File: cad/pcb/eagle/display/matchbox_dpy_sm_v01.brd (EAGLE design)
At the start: 40 x 32 mm, 16 parts, among them J1 DF12-32-DS, J2 DF12-32-DS, SW1 B3U-3100PM-B, U1 LM2750

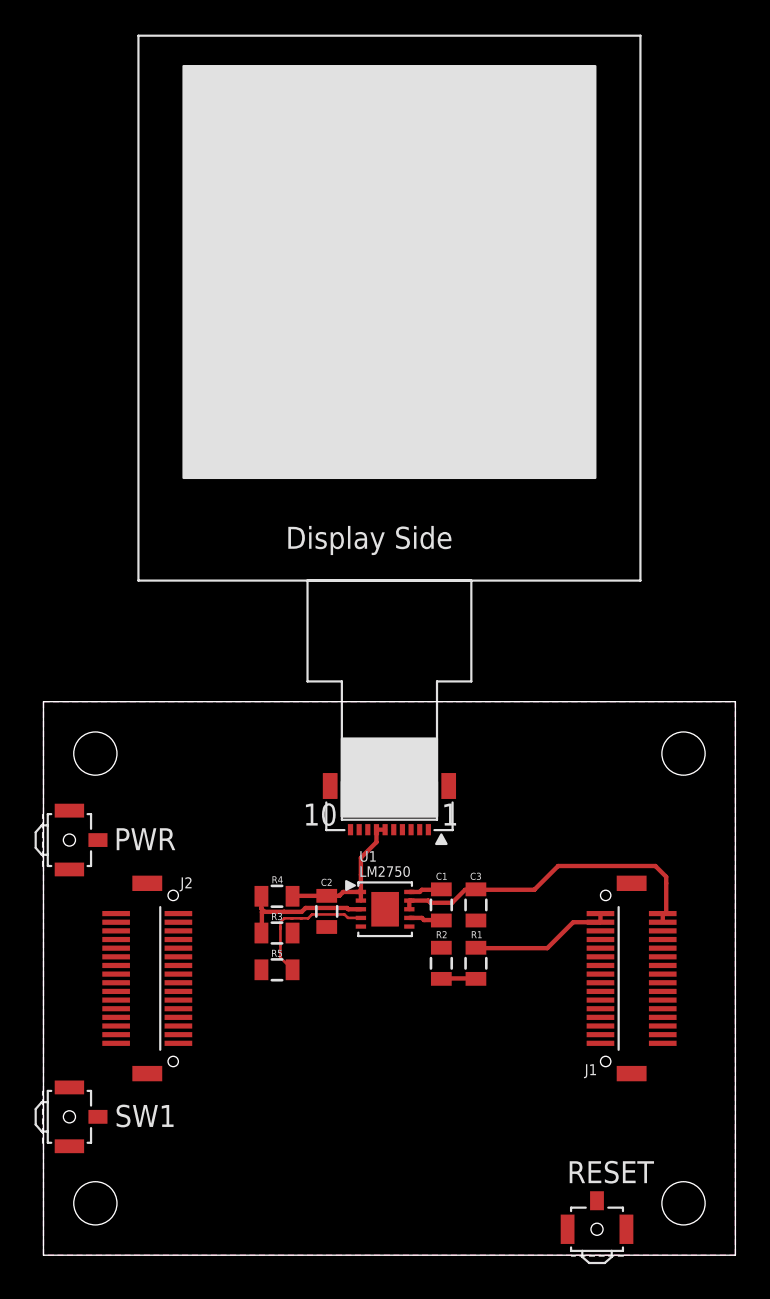
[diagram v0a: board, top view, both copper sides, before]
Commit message: Tweak display board v01
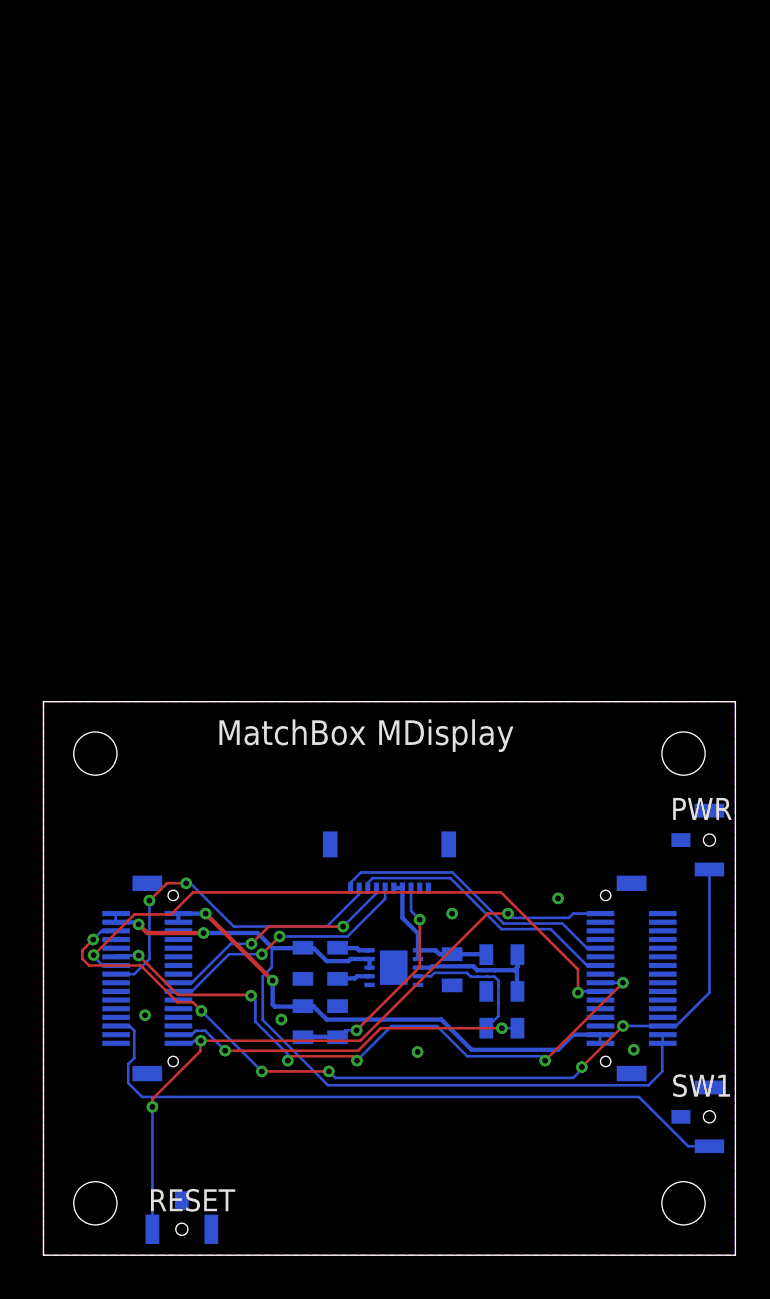
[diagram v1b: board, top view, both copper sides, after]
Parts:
- moved PWR 37.0 mm to (38.5, 24.0), flipped to the bottom
- moved SW1 37.0 mm to (38.5, 8.00), flipped to the bottom
- moved J1 28.0 mm to (6.00, 16.0), flipped to the bottom
- moved J2 28.0 mm to (34.0, 16.0), flipped to the bottom
- moved RESET 24.0 mm to (8.00, 1.50), flipped to the bottom
- moved R3 13.4 mm to (26.5, 15.2), flipped to the bottom
- moved R4 13.4 mm to (26.5, 17.4), flipped to the bottom
- moved R5 13.4 mm to (26.5, 13.1), flipped to the bottom
- moved C3 10.6 mm to (15.0, 16.9), flipped to the bottom
- moved R1 10.6 mm to (15.0, 13.5), flipped to the bottom
- moved C2 8.00 mm to (23.6, 16.5), flipped to the bottom
- moved C1 6.88 mm to (17.0, 16.9), flipped to the bottom
- moved R2 6.88 mm to (17.0, 13.5), flipped to the bottom
- moved U$1 3.50 mm to (20.0, 35.5), flipped to the bottom
- moved U1 3.41 mm to (20.2, 16.6), flipped to the bottom
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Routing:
- net PWR_ON: track 0.00 -> 51.3 mm, vias 0 -> 6
- net RESET#: track 0.00 -> 39.9 mm, vias 0 -> 3
- net PC13: track 0.00 -> 39.4 mm
- net PC5: track 0.00 -> 37.9 mm, vias 0 -> 6
- net PC4: track 0.00 -> 35.6 mm, vias 0 -> 2
- net VCC: track 19.5 -> 48.2 mm, vias 0 -> 2
- net VCC_3V3: track 8.35 -> 29.9 mm, vias 0 -> 2
- net PB9: track 0.00 -> 20.7 mm, vias 0 -> 2
- net PC3: track 0.00 -> 20.4 mm, vias 0 -> 2
- net PB10: track 0.00 -> 16.8 mm
- net PB1: track 0.00 -> 16.0 mm
- net PB5: track 0.00 -> 14.8 mm, vias 0 -> 2
- net PB4: track 0.00 -> 13.9 mm, vias 0 -> 2
- net EXTMODE: track 2.05 -> 13.2 mm, vias 0 -> 2
